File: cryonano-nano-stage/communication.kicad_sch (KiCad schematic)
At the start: 40 parts, among them J6 RJ45_Hanrun_HR911105A_Horizon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, J7 10118194-0001LF, U10 LAN8742A, U5 ECMF02-2AMX6, U9 USBLC6-4SC6, Y3 25.0MHz

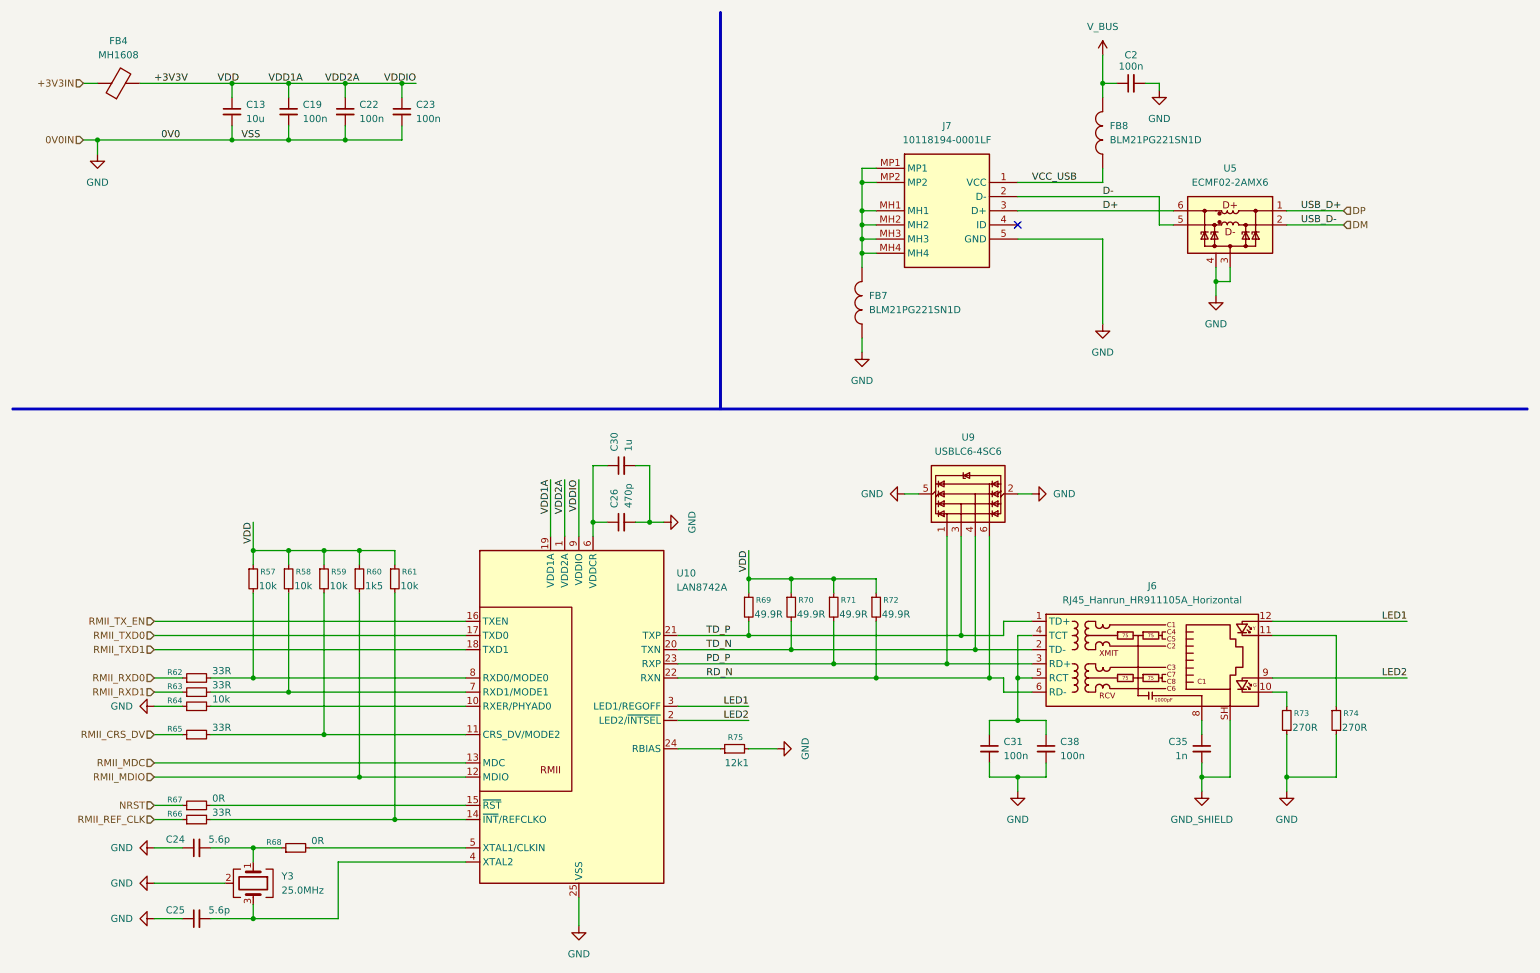
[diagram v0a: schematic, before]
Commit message: sch improved
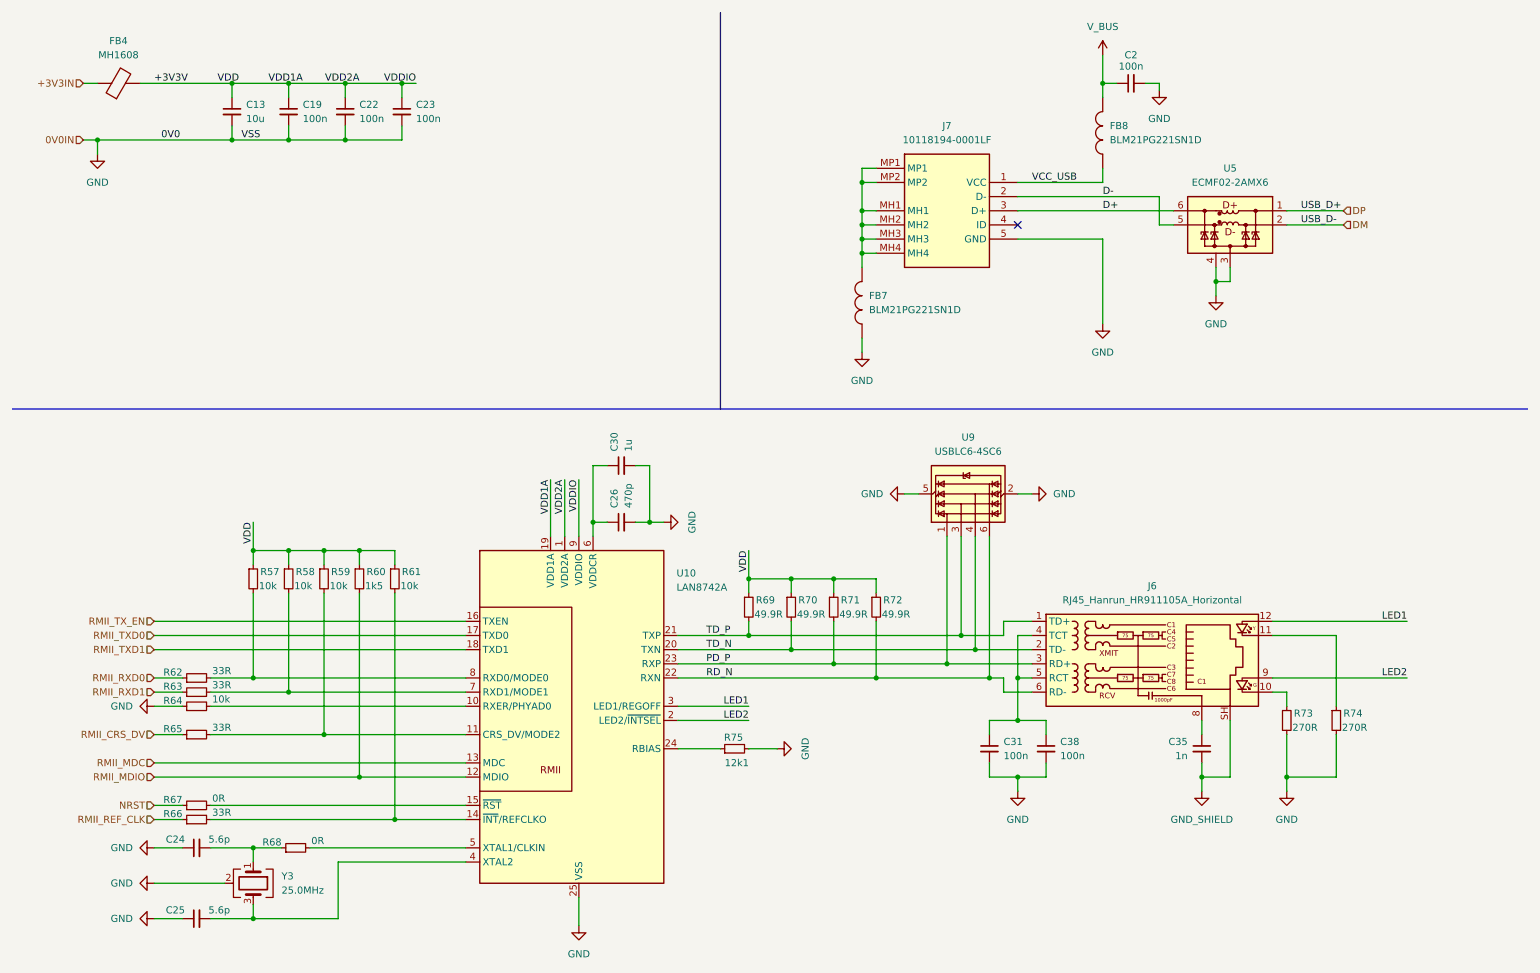
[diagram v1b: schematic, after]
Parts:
- U10: footprint Package_DFN_QFN:VQFN-24-1EP_4x4mm_P0.5mm_EP2.5x2.5mm_ThermalVias -> footprints:VQFN-24-1EP_4x4mm_P0.5mm_EP2.5x2.5mm_ThermalVias
